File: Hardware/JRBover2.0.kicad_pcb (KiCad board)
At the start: 2 copper layers, 46 x 45 mm, 25 parts, among them J1 EncoderMotorDerecha, J10 Input of Driver L9110, J2 HC_SRO4, J3 HC_SRO4, J4 HC_SRO4, J5 CableAlimentacion, J6 SWITCH, J7 Programador, J8 BOTON, J9 EncoderMotorIzquierda, U1 ESP32-WROOM-32, U2 L7805, U3 LM1117-SOT

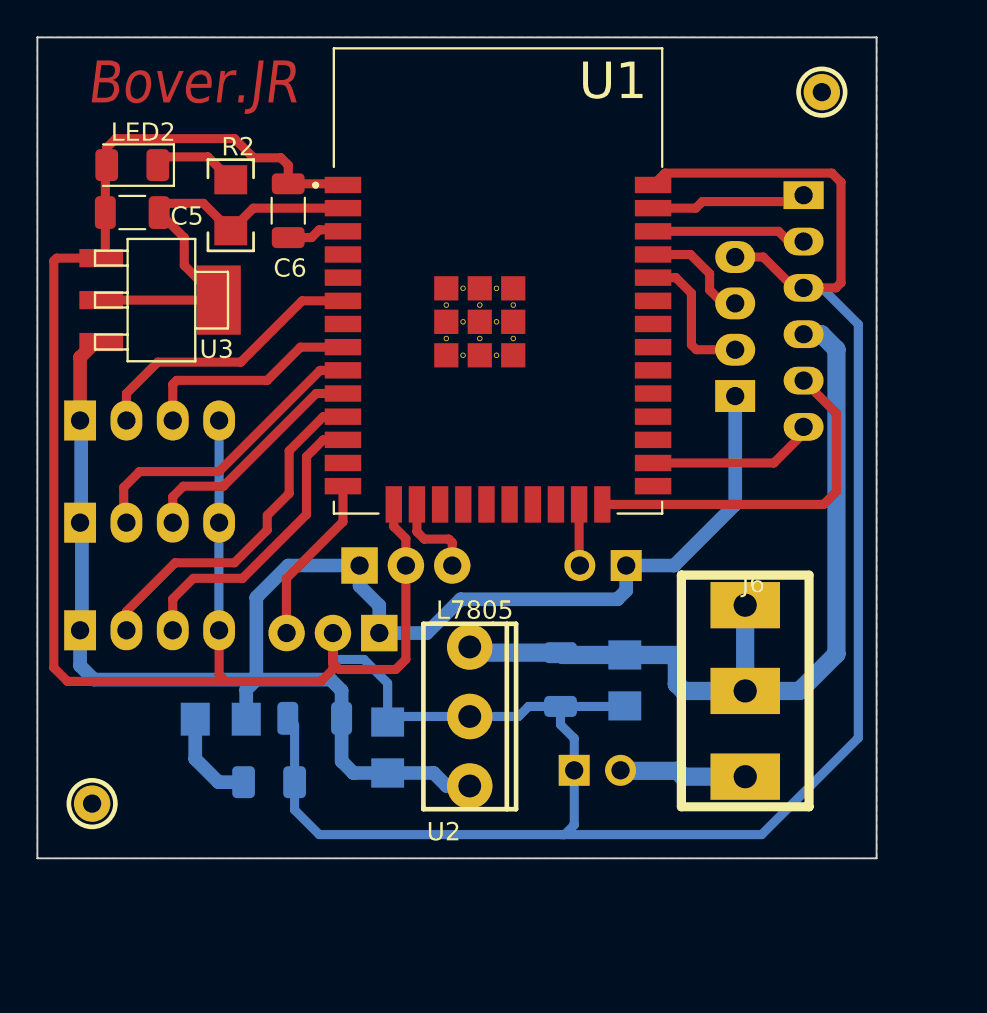
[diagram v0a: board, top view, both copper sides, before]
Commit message: Placa corregida por Bustos siuuuuuuuuuuuuuuuuuuuuuu
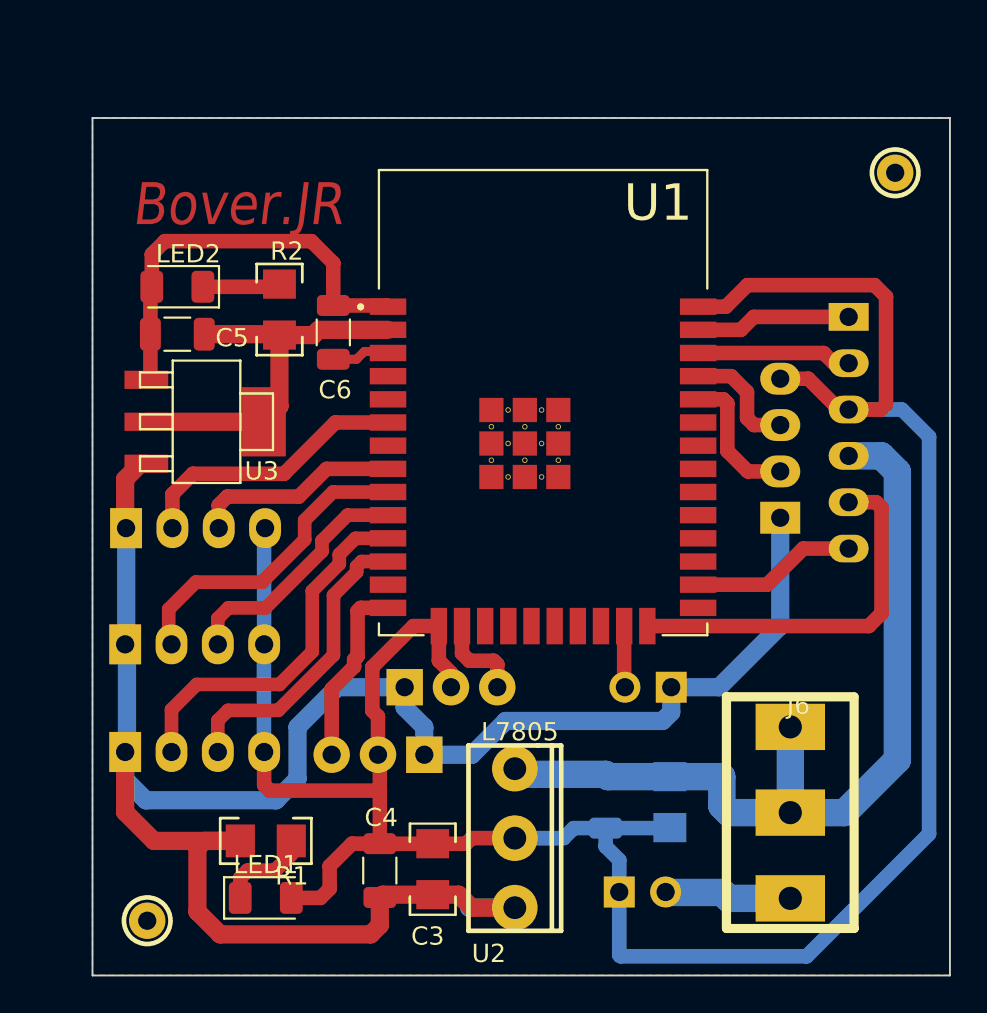
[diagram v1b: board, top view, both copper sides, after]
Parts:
- C3, C4, LED1, R1: moved to F.Cu
- moved C4 9.08 mm to (134.8, 120.7), turned to -90 degrees
- moved R1 7.11 mm to (128.5, 119.0), turned to 0 degrees
- moved C1 7.11 mm to (150.7, 116.9)
- moved C2 7.11 mm to (147.1, 116.9)
- moved C3 7.11 mm to (137.7, 120.6)
- moved C5 7.11 mm to (123.7, 91.3)
- moved C6 7.11 mm to (132.2, 91.2)
- moved J10 7.11 mm to (160.5, 96.7)
- moved J3 7.11 mm to (124.6, 108.3)
- moved J4 7.11 mm to (124.6, 114.2)
- moved J5 7.11 mm to (147.9, 121.8)
- moved J6 7.11 mm to (157.3, 117.5)
- moved J7 7.11 mm to (156.7, 97.5)
- moved J8 7.11 mm to (150.7, 110.6)
- moved J9 7.11 mm to (138.7, 110.6)
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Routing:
- net GND: track 209.6 -> 162.3 mm
- net +5V: track 91.5 -> 110.3 mm
- net +3V3: track 24.0 -> 21.8 mm
- net +7.5V: track 46.4 -> 47.6 mm
- net /Echo3: track 19.2 -> 20.3 mm
- net /IN2: track 20.0 -> 20.8 mm
- net /D0: track 9.34 -> 10.2 mm
- net /Trig1: track 12.2 -> 11.4 mm
- net /Echo2: track 16.7 -> 17.3 mm
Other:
- board size 46 x 45 mm -> 47 x 47 mm
